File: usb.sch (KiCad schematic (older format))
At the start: 21 parts, among them J3 JTAG, P1 USB_OTG, U1 LFE5U-85F-6BG381C, Y1 FNETHE025

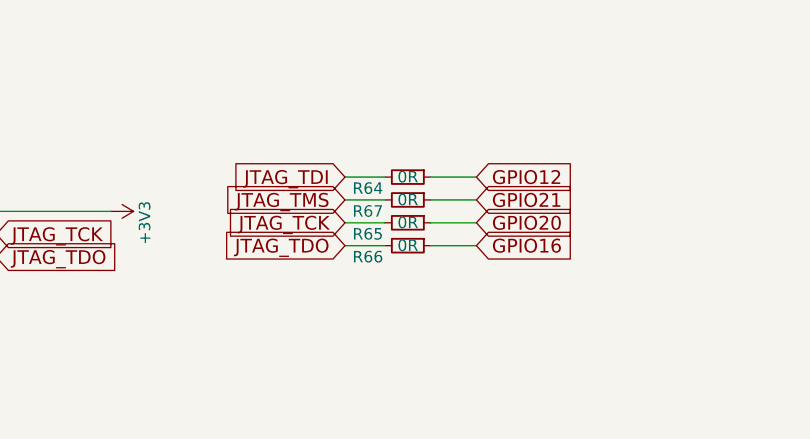
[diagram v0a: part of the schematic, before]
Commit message: Changing GPIO>>JTAG reseistor to connector
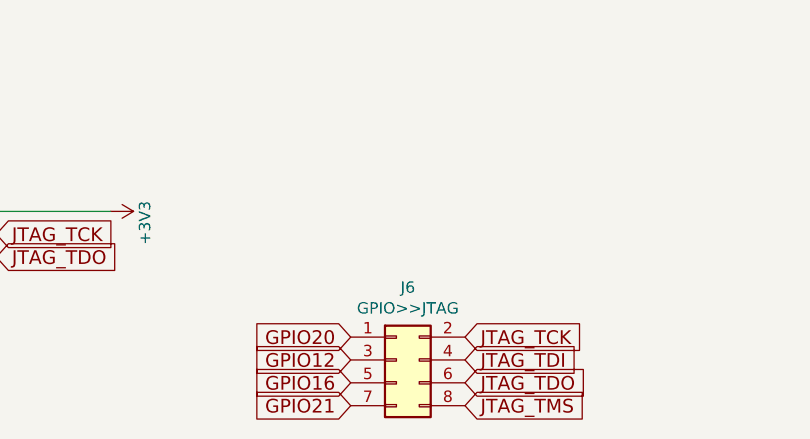
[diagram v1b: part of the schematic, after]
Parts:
- removed R64, R65, R66, R67: 0R, Resistor_SMD:R_0201_0603Metric, symbol Device:R_Small
- added J6: GPIO>>JTAG, Connector_PinHeader_1.00mm:PinHeader_2x04_P1.00mm_Vertical, symbol Connector_Generic:Conn_02x04_Odd_Even
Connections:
- net GPIO12: now also J6.3 (Pin_3)
- net GPIO16: now also J6.5 (Pin_5)
- net GPIO20: now also J6.1 (Pin_1)
- net GPIO21: now also J6.7 (Pin_7)
- net JTAG_TCK: now also J6.2 (Pin_2)
- net JTAG_TDI: now also J6.4 (Pin_4)
- net JTAG_TDO: now also J6.6 (Pin_6)
- net JTAG_TMS: now also J6.8 (Pin_8)
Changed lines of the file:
@@
 Wire Wire Line
 	7550 5500 7600 5500
-Text GLabel 9125 5150 0    60   Input ~ 0
+Text GLabel 9650 5950 2    60   Input ~ 0
 JTAG_TDI
-Text GLabel 9125 5250 0    60   Input ~ 0
+Text GLabel 9650 6150 2    60   Input ~ 0
 JTAG_TMS
-Text GLabel 9125 5350 0    60   Input ~ 0
+Text GLabel 9650 5850 2    60   Input ~ 0
 JTAG_TCK
-Text GLabel 9125 5450 0    60   Input ~ 0
+Text GLabel 9650 6050 2    60   Input ~ 0
 JTAG_TDO
-Text GLabel 9700 5450 2    60   Input ~ 0
+Text GLabel 9150 6050 0    60   Input ~ 0
 GPIO16
-Text GLabel 9700 5350 2    60   Input ~ 0
+Text GLabel 9150 5850 0    60   Input ~ 0
 GPIO20
-Text GLabel 9700 5250 2    60   Input ~ 0
+Text GLabel 9150 6150 0    60   Input ~ 0
 GPIO21
-Text GLabel 9700 5150 2    60   Input ~ 0
+Text GLabel 9150 5950 0    60   Input ~ 0
 GPIO12
 Text GLabel 5250 5100 0    60   Input ~ 0
@@
 Text GLabel 6600 3775 0    50   Output ~ 0
 RGMII_RXD2
-$Comp
-L Device:R_Small R64
-U 1 1 648C922E
-P 9400 5150
-F 0 "R64" V 9450 4975 50  0000 C CNN
-F 1 "0R" V 9400 5150 50  0000 C CNN
-F 2 "Resistor_SMD:R_0201_0603Metric" H 9400 5150 50  0001 C CNN
-F 3 "~" H 9400 5150 50  0001 C CNN
-	1    9400 5150
-	0    1    1    0
-$EndComp
-$Comp
-L Device:R_Small R65
-U 1 1 64928528
-P 9400 5350
-F 0 "R65" V 9450 5175 50  0000 C CNN
-F 1 "0R" V 9400 5350 50  0000 C CNN
-F 2 "Resistor_SMD:R_0201_0603Metric" H 9400 5350 50  0001 C CNN
-F 3 "~" H 9400 5350 50  0001 C CNN
-	1    9400 5350
-	0    1    1    0
-$EndComp
-$Comp
-L Device:R_Small R66
-U 1 1 649432D8
-P 9400 5450
-F 0 "R66" V 9450 5275 50  0000 C CNN
-F 1 "0R" V 9400 5450 50  0000 C CNN
-F 2 "Resistor_SMD:R_0201_0603Metric" H 9400 5450 50  0001 C CNN
-F 3 "~" H 9400 5450 50  0001 C CNN
-	1    9400 5450
-	0    1    1    0
-$EndComp
-$Comp
-L Device:R_Small R67
-U 1 1 64976EC1
-P 9400 5250
-F 0 "R67" V 9450 5075 50  0000 C CNN
-F 1 "0R" V 9400 5250 50  0000 C CNN
-F 2 "Resistor_SMD:R_0201_0603Metric" H 9400 5250 50  0001 C CNN
-F 3 "~" H 9400 5250 50  0001 C CNN
-	1    9400 5250
-	0    1    1    0
-$EndComp
-Wire Wire Line
-	9125 5150 9300 5150
-Wire Wire Line
-	9125 5250 9300 5250
-Wire Wire Line
-	9125 5350 9300 5350
-Wire Wire Line
-	9125 5450 9300 5450
-Wire Wire Line
-	9500 5150 9700 5150
-Wire Wire Line
-	9500 5250 9700 5250
-Wire Wire Line
-	9500 5350 9700 5350
-Wire Wire Line
-	9500 5450 9700 5450
 Text GLabel 10825 2350 2    60   Input ~ 0
 GPIO12
@@
 Wire Wire Line
 	7900 2250 8650 2250
+$Comp
+L Connector_Generic:Conn_02x04_Odd_Even J6
+U 1 1 64CCAF42
+P 9350 5950
+F 0 "J6" H 9400 6267 50  0000 C CNN
+F 1 "GPIO>>JTAG" H 9400 6176 50  0000 C CNN
+F 2 "Connector_PinHeader_1.00mm:PinHeader_2x04_P1.00mm_Vertical" H 9350 5950 50  0001 C CNN
+F 3 "~" H 9350 5950 50  0001 C CNN
+	1    9350 5950
+	1    0    0    -1
+$EndComp
 $EndSCHEMATC
